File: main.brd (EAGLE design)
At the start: 74.9 x 37.6 mm, 7 parts

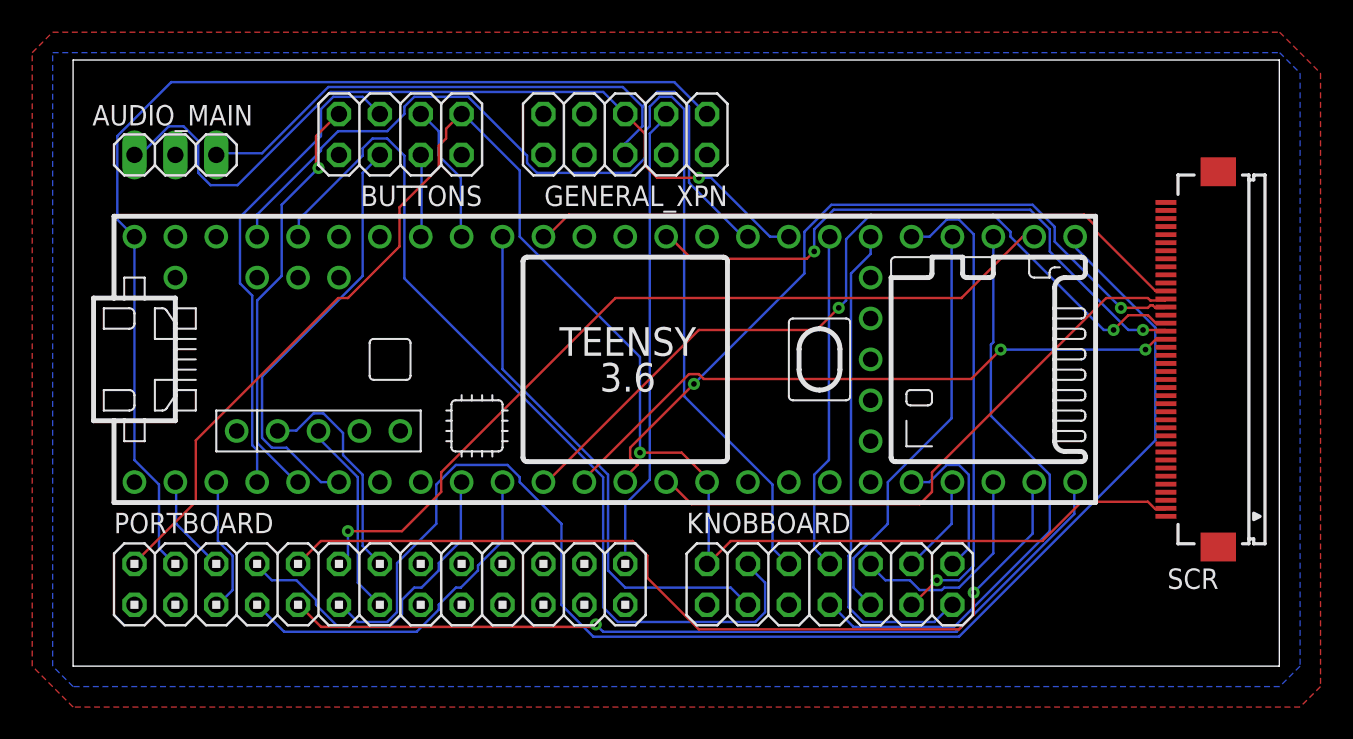
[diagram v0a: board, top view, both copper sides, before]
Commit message: PDFs of sch & brd
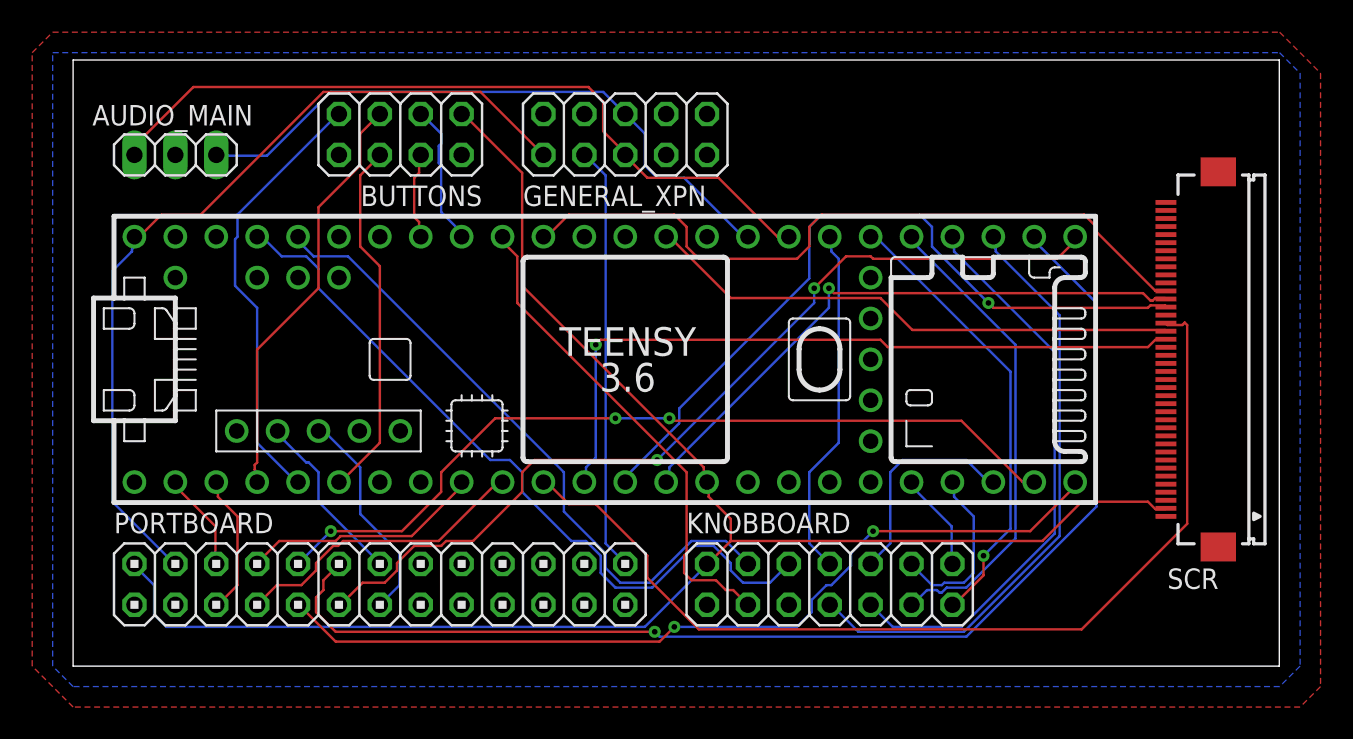
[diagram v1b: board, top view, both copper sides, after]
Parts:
- turned GENERAL_XPN to 0 degrees
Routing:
- net MIDIOUT4: track 85.8 -> 57.0 mm, vias 0 -> 2
- net JOYSTICK_X: track 68.4 -> 46.9 mm
- net MIDIIN4: track 53.2 -> 74.4 mm
- net JOYSTICK_Y: track 57.7 -> 40.7 mm
- net +5V: track 66.9 -> 53.3 mm
- net ROTENC4_A: track 25.9 -> 35.5 mm
- net SCR_DC: track 51.5 -> 61.1 mm, vias 2 -> 0
- net MIDIIN2: track 21.2 -> 15.0 mm
- net AUDIO_R: track 45.6 -> 39.6 mm
- net ROTENC1_B: track 6.16 -> 11.0 mm
- net SCR_CS: track 40.2 -> 44.8 mm, vias 2 -> 1
- net SCR_CLK: track 37.6 -> 33.5 mm, vias 2 -> 0
- net BUTTON_DATA: track 26.5 -> 22.4 mm
- net ROTENC1_A: track 10.2 -> 6.16 mm
- net MIDIIN3: track 55.9 -> 51.8 mm, vias 1 -> 3
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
